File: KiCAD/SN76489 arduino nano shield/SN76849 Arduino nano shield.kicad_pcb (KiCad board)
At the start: 2 copper layers, 74 x 52.9 mm, 12 parts, among them J2 audio_debug, J3 OLED_wit, J5 LOGO, J6 gat1, J7 gat2, J8 geluid_uit, U1 PCF8574, U3 SN76489

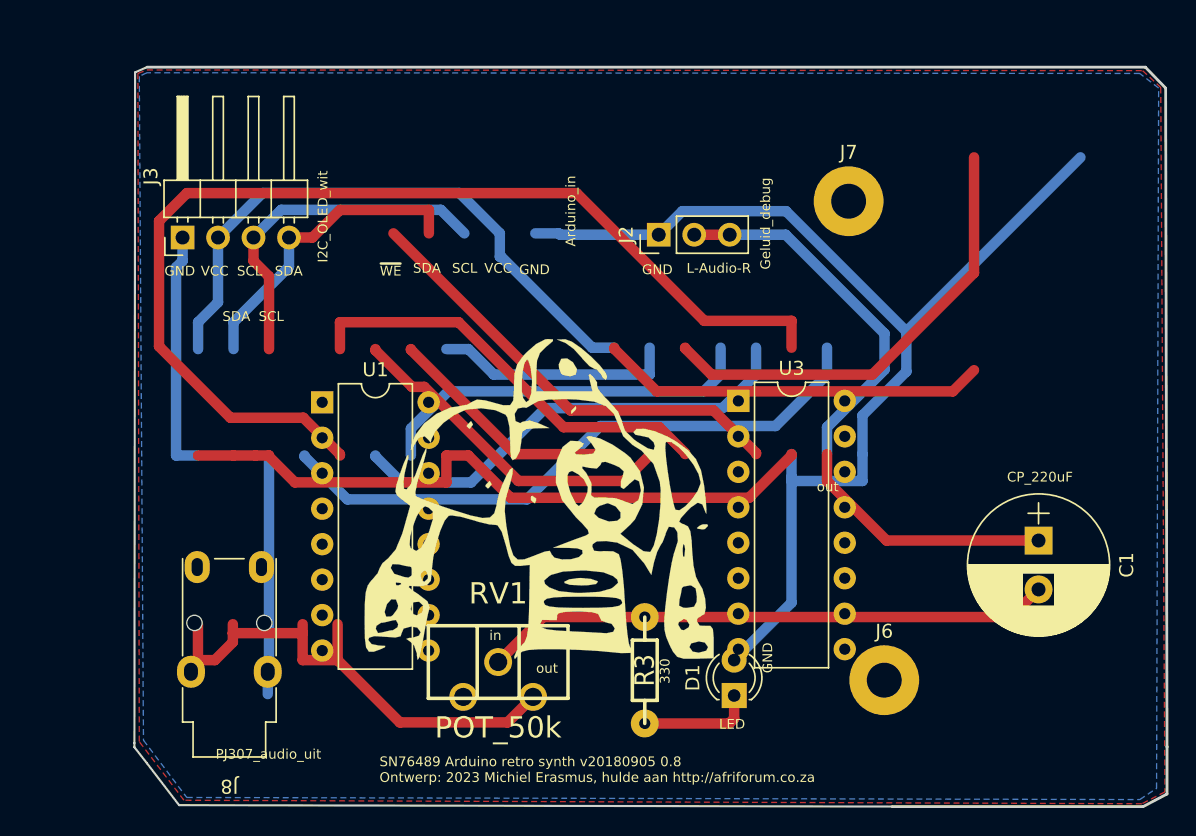
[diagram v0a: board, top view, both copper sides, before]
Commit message: Bijgewerkt
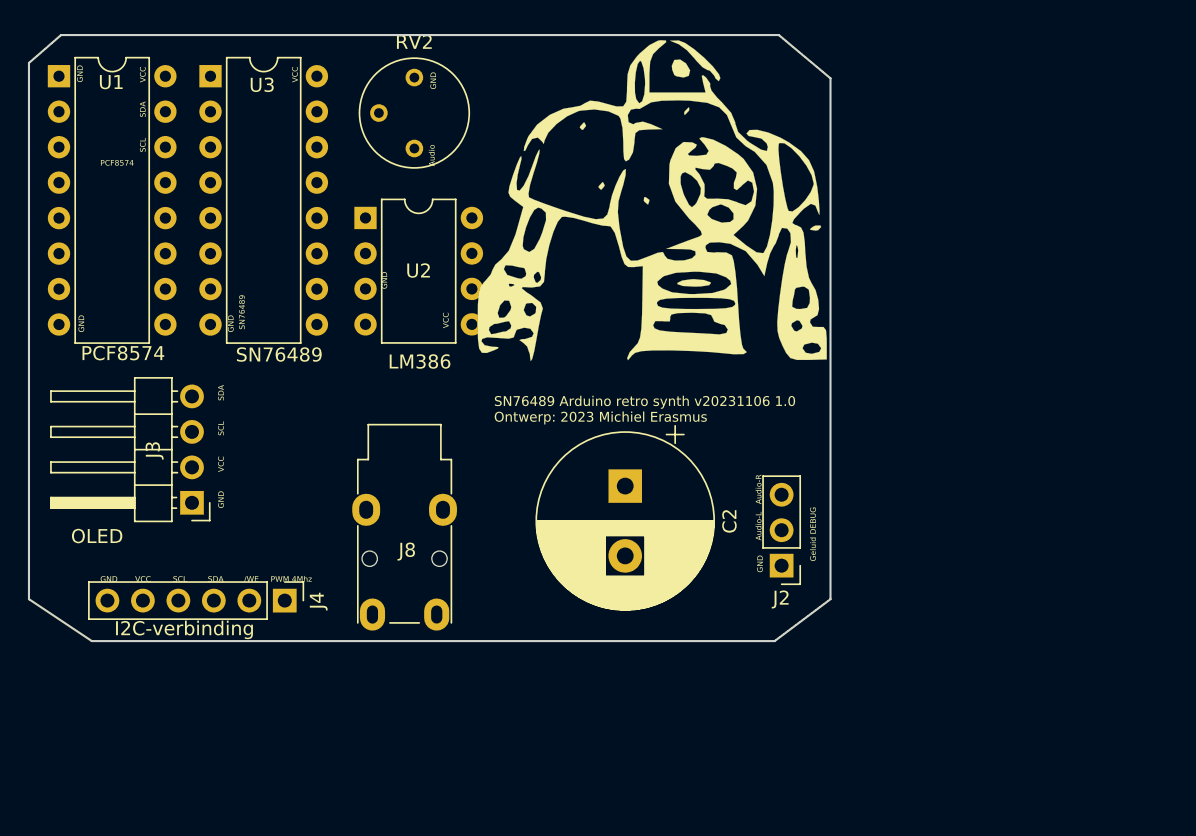
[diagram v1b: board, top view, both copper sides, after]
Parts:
- removed C1: CP_220uF, Capacitors_THT:CP_Radial_D10.0mm_P3.50mm
- removed D1: Liggie, LEDs:LED_D3.0mm
- removed J6: gat1, Mounting_Holes:MountingHole_2.5mm_Pad
- removed J7: gat2, Mounting_Holes:MountingHole_2.5mm_Pad
- removed R3: R1k, w_pth_resistors:RC03
- removed RV1: POT_50k, w_pth_resistors:trimmer_ecp_ca9-h2,5
- added C2: 250uF, Capacitor_THT:CP_Radial_D12.5mm_P5.00mm, F.Cu at (69.4, 52.9)
- added J4: ESP32Conn, Connector_PinHeader_2.54mm:PinHeader_1x06_P2.54mm_Vertical, F.Cu at (45.0, 61.1)
- added RV2: Pot_10k, Potentiometer_THT:Potentiometer_Bourns_3339P_Vertical, F.Cu at (54.3, 28.7)
- added U2: LM386, Package_DIP:DIP-8_W7.62mm, F.Cu at (50.8, 33.7)
- moved U3 44.4 mm to (39.7, 23.6)
- moved U1 30.0 mm to (28.9, 23.6)
- moved J2 25.3 mm to (80.6, 58.6), turned to 180 degrees
- moved J5 22.9 mm to (71.4, 32.2)
- moved J3 19.0 mm to (38.4, 54.1), turned to 180 degrees
- moved J8 13.6 mm to (50.9, 54.6), turned to 0 degrees
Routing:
- net GND: track 241.5 -> 0.00 mm
- net /VCC: track 123.7 -> 0.00 mm
- net /Audio: track 45.7 -> 0.00 mm
- net /P0: track 44.4 -> 0.00 mm
- net Net-(C1-Pad2): track 40.9 -> 0.00 mm
- net Net-(J8-Pad2): track 36.2 -> 0.00 mm
- net /P2: track 33.2 -> 0.00 mm
- net /Clock: track 32.8 -> 0.00 mm
- net /~{WE}: track 32.6 -> 0.00 mm
- net /P7: track 30.6 -> 0.00 mm
- net /SCL: track 25.1 -> 0.00 mm
- net /SDA: track 22.1 -> 0.00 mm
- net /P5: track 17.7 -> 0.00 mm
- net /P4: track 17.2 -> 0.00 mm
- net Net-(D1-K): track 8.19 -> 0.00 mm
- removed copper zone on B.Cu, net GND
- removed copper zone on F.Cu, net GND
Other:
- board size 74 x 52.9 mm -> 57.4 x 43.4 mm
- board text added: "/WE"
- board text added: "Audio"
- board text added: "Audio-L"
- board text added: "Audio-R"
- board text added: "Geluid DEBUG"
- board text added: "I2C-verbinding"
- board text added: "LM386"
- board text added: "OLED"
- board text added: "PCF8574"
- board text added: "PWM 4Mhz"
- board text added: "SN76489"
- board text added: "SN76489 Arduino retro synth v20231106 1.0 Ontwerp: 2023 Michiel Erasmus"
- board text removed: "330"
- board text removed: "Arduino_in"
- board text removed: "CP_220uF"
- board text removed: "Geluid_debug"
- board text removed: "I2C_OLED_wit"
- board text removed: "L-Audio-R"
- board text removed: "LED"
- board text removed: "PJ307_audio_uit"
- board text removed: "SN76489 Arduino retro synth v20180905 0.8 Ontwerp: 2023 Michiel Erasmus, hulde aan http://afriforum.co.za"
- board text removed: "in"
- board text removed: "out"
- board text removed: "~{WE}"
